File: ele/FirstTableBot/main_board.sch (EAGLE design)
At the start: 164 parts, among them IC3 CP2102N-28, T1 BC337, T2 BC337, U1 ESP-WROOM-32, U2 UM18533, X3 USB-MICRO-B-BOTTOM, X4 POWER_IN

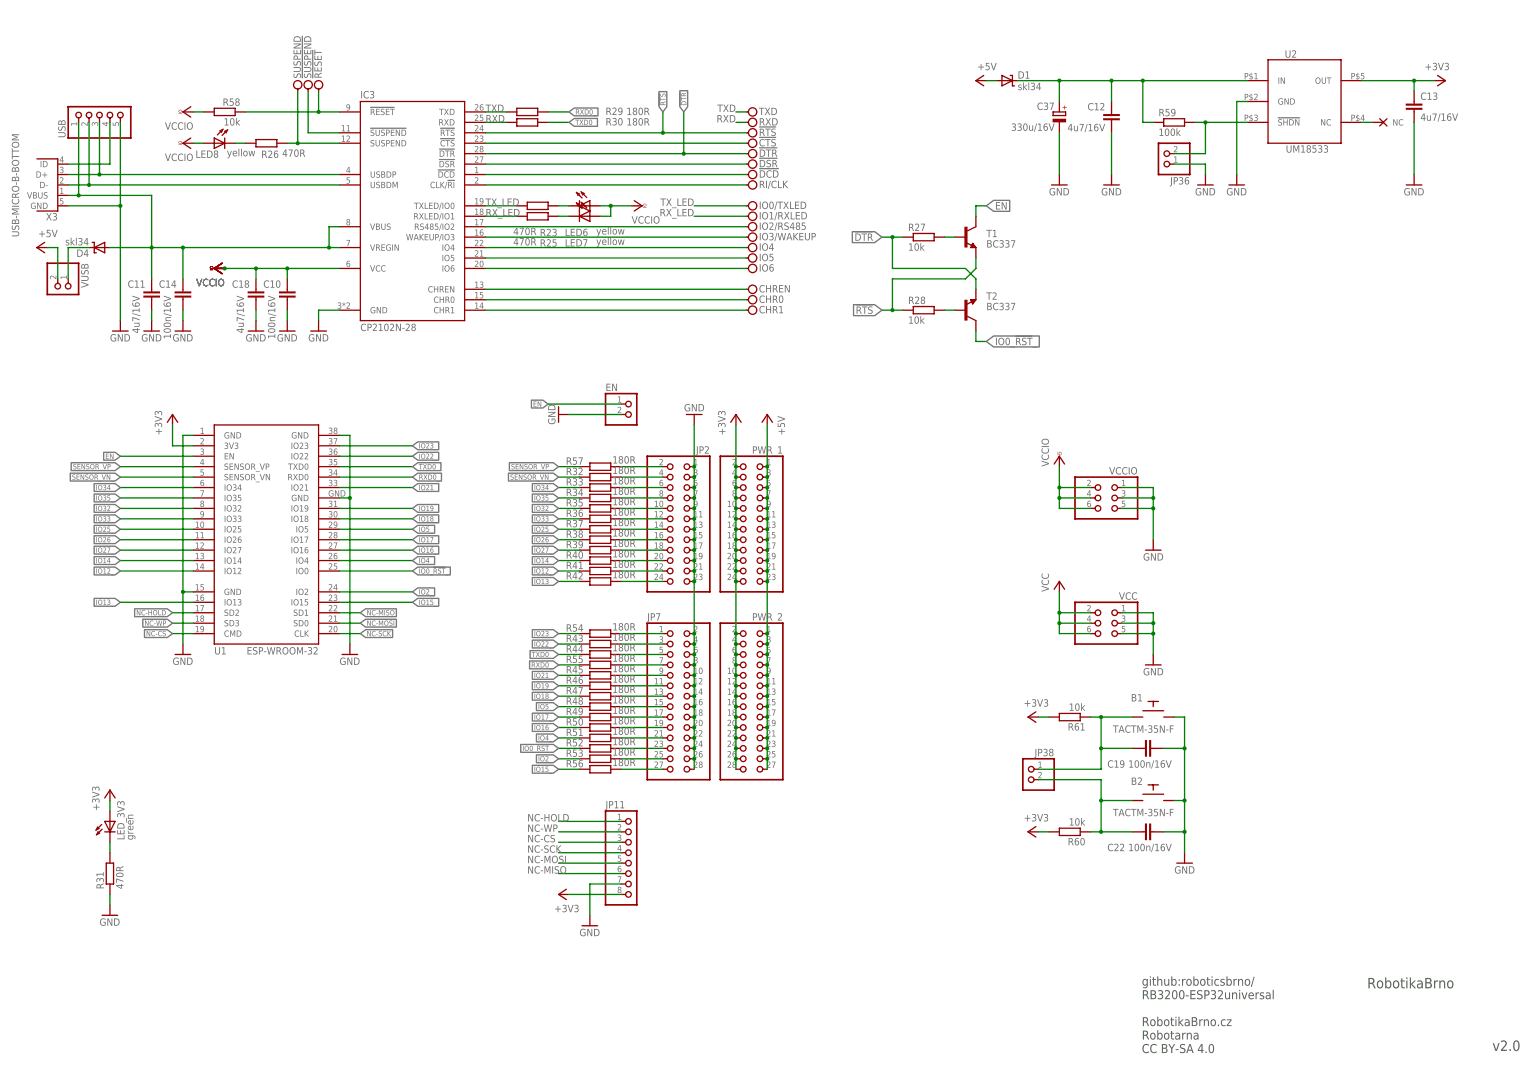
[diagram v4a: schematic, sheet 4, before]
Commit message: mereni proudu
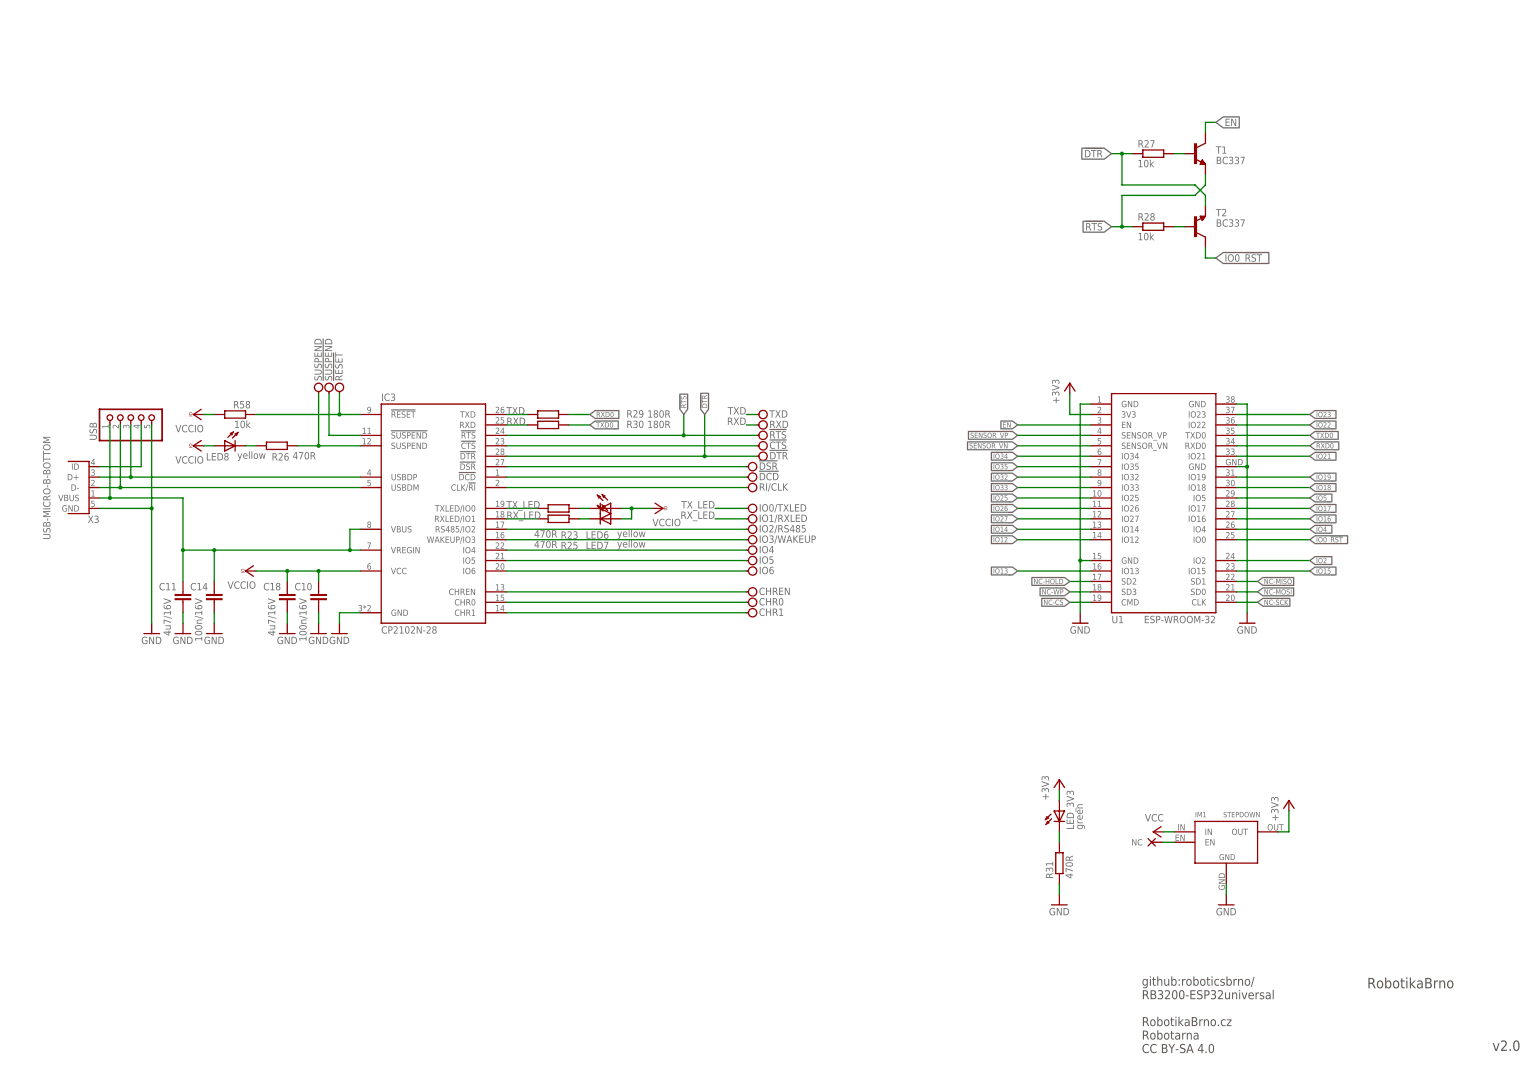
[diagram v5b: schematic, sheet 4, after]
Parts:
- removed B1, B2: TACTM-35N-F, TACTM-35N-F:TACTM-35N-F
- removed C12, C13: 4u7/16V, rcl_upravena:C-EUC0603
- removed C19, C22: 100n/16V, rcl_upravena:C-EUC0402
- removed C37: 330u/16V, rcl_upravena:CPOL-EUE5-10.5
- removed D1, D4: skl34, diode:SHOTTKY-SOD123
- removed EN, JP36, JP38, VUSB: (no value), pinhead:PINHD-1X2
- removed JP11: (no value), pinhead:PINHD-1X8
- removed JP2, PWR_1: (no value), pinhead:PINHD-2X12
- removed JP7, PWR_2: (no value), pinhead:PINHD-2X14
- removed NC7: NC, NC:NC
- removed R32, R33, R34, R35, R36, R37, R38, R39, R40, R41, R42, R43, R44, R45, R46, R47, R48, R49, R50, R51, R52, R53, R54, R55, R56, R57: 180R, rcl_upravena:R-EU_R0603
- removed R59: 100k, rcl_upravena:R-EU_R0603
- removed R60, R61: 10k, rcl_upravena:R-EU_R0603
- removed U2: UM18533, um185xx:UM185XX
- removed VCC, VCCIO: (no value), pinhead:PINHD-2X3
- added IM1: STEPDOWN, StepDown:STEPDOWN
- added NC2: NC, NC:NC
- added R19, R62: (no value), resistor:R-EU_M1206
- added U$11: BA10358F-E2SOIC, Rohm:BA10358F-E2SOIC
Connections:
- removed net !SHDN: JP36.2, R59.2, U2.!SHDN
- removed net 3V3_IN: C12.1, C37.+, D1.C, R59.1, U2.IN
- removed net 5V_USB: D4.C, VUSB.1
- removed net BTN0: B1.P$4, C19.2, JP38.1, R61.1
- removed net BTN1: B2.P$4, C22.2, JP38.2, R60.1
- removed net IO0_!RST: JP7.23, R52.1
- removed net IO12: JP2.22, R41.1
- removed net IO13: JP2.24, R42.1
- removed net IO14: JP2.20, R40.1
- removed net IO15: JP7.27, R56.1
- removed net IO16: JP7.19, R50.1
- removed net IO17: JP7.17, R49.1
- removed net IO18: JP7.13, R47.1
- removed net IO19: JP7.11, R46.1
- removed net IO2: JP7.25, R53.1
- removed net IO21: JP7.9, R45.1
- removed net IO22: JP7.3, R43.1
- removed net IO23: JP7.1, R54.1
- removed net IO25: JP2.14, R37.1
- removed net IO26: JP2.16, R38.1
- removed net IO27: JP2.18, R39.1
- removed net IO32: JP2.10, R35.1
- removed net IO33: JP2.12, R36.1
- removed net IO34: JP2.6, R33.1
- removed net IO35: JP2.8, R34.1
- removed net IO4: JP7.21, R51.1
- removed net IO5: JP7.15, R48.1
- removed net RXD0: JP7.7, R55.1
- removed net SENSOR_VN: JP2.4, R32.1
- removed net SENSOR_VP: JP2.2, R57.1
- removed net TXD0: JP7.5, R44.1
- removed net U2_NC: NC7.NC, U2.NC
- new net AMPLIFIED_I-MOT_A: U$11.OUT2
- new net AMPLIFIED_I-MOT_B: U$11.OUT1
- new net I-MOT_A: R19.2, U$11.+IN2, U$9.AISEN
- new net I-MOT_B: R62.2, U$11.+IN1, U$9.BISEN
- new net IO9_NC1: IM1.EN, NC2.NC
- net +3V3: now also IM1.OUT; no longer C13.1, JP11.8, PWR_1.10, PWR_1.12, PWR_1.14, PWR_1.16, PWR_1.18, PWR_1.2, PWR_1.20, PWR_1.22, PWR_1.24, PWR_1.4, PWR_1.6, PWR_1.8, PWR_2.10, PWR_2.12, PWR_2.14, PWR_2.16, PWR_2.18, PWR_2.2, PWR_2.20, PWR_2.22, PWR_2.24, PWR_2.26, PWR_2.28, PWR_2.4, PWR_2.6, PWR_2.8, R60.2, R61.2, U2.OUT
- net +5V: no longer D1.A, PWR_1.1, PWR_1.11, PWR_1.13, PWR_1.15, PWR_1.17, PWR_1.19, PWR_1.21, PWR_1.23, PWR_1.3, PWR_1.5, PWR_1.7, PWR_1.9, PWR_2.1, PWR_2.11, PWR_2.13, PWR_2.15, PWR_2.17, PWR_2.19, PWR_2.21, PWR_2.23, PWR_2.25, PWR_2.27, PWR_2.3, PWR_2.5, PWR_2.7, PWR_2.9, VUSB.2
- net EN: no longer EN.1
- net GND: now also IM1.GND, R19.1, R62.1, U$11.-IN1, U$11.-IN2, U$11.VEE; no longer B1.P$3, B2.P$3, C12.2, C13.2, C19.1, C22.1, C37.-, EN.2, JP11.7, JP2.1, JP2.11, JP2.13, JP2.15, JP2.17, JP2.19, JP2.21, JP2.23, JP2.3, JP2.5, JP2.7, JP2.9, JP36.1, JP7.10, JP7.12, JP7.14, JP7.16, JP7.18, JP7.2, JP7.20, JP7.22, JP7.24, JP7.26, JP7.28, JP7.4, JP7.6, JP7.8, U$9.AISEN, U$9.BISEN, U2.GND, VCC.1, VCC.3, VCC.5, VCCIO.1, VCCIO.3, VCCIO.5
- net IO0_!RST!_: no longer R52.2
- net IO12_: no longer R41.2
- net IO13_: no longer R42.2
- net IO14_: no longer R40.2
- net IO15_: no longer R56.2
- net IO16_: no longer R50.2
- net IO17_: no longer R49.2
- net IO18_: no longer R47.2
- net IO19_: no longer R46.2
- net IO21_: no longer R45.2
- net IO22_: no longer R43.2
- net IO23_: no longer R54.2
- net IO25_: no longer R37.2
- net IO26_: no longer R38.2
- net IO27_: no longer R39.2
- net IO2_: no longer R53.2
- net IO32_: no longer R35.2
- net IO33_: no longer R36.2
- net IO34_: no longer R33.2
- net IO35_: no longer R34.2
- net IO4_: no longer R51.2
- net IO5_: no longer R48.2
- net NC-CS: no longer JP11.3
- net NC-HOLD: no longer JP11.1
- net NC-MISO: no longer JP11.6
- net NC-MOSI: no longer JP11.5
- net NC-SCK: no longer JP11.4
- net NC-WP: no longer JP11.2
- net RXD0_: no longer R55.2
- net SENSOR_VN_: no longer R32.2
- net SENSOR_VP_: no longer R57.2
- net TXD0_: no longer R44.2
- net VCC: now also IM1.IN, U$11.VCC; no longer VCC.2, VCC.4, VCC.6
- net VCCIO: no longer VCCIO.2, VCCIO.4, VCCIO.6
- net VUSB: no longer D4.A
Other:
- moved on the sheet: C10, C11, C14, C18, C23, C6, C7, CHR0, CHR1, CHREN, D3, IC3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

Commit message: ir led pro encodery
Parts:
- removed !CTS, !DCD, !DSR, !DTR, !RESET, !RTS, !SUSPEND, CHR0, CHR1, CHREN, IO0/TXLED, IO1/RXLED, IO2/RS485, IO3/WAKEUP, IO4, IO5, IO6, RI/CLK, RXD, SUSPEND, TXD: PINH1X01, pinhead_smd:PINH1X01
- removed C10, C14: 100n/16V, rcl_upravena:C-EUC0402
- removed C11, C18: 4u7/16V, rcl_upravena:C-EUC0603
- removed IC3: CP2102N-28, CP2102N:CP2102N-28
- removed IM1: STEPDOWN, StepDown:STEPDOWN
- removed JP1: PINH2X06, pinhead_smd:PINH2X06
- removed LED6, LED7, LED8: yellow, led:LEDCHIP-LED0603
- removed LED_3V3: green, led:LEDCHIPLED_0603
- removed NC2: NC, NC:NC
- removed R29, R30: 180R, rcl_upravena:R-EU_R0603
- removed R31: 470R, rcl_upravena:R-EU_R0603
- removed R58: 10k, rcl_upravena:R-EU_R0603
- removed RN1: (no value), resistor-dil:2R-NEXB24V
- removed T1, T2: BC337, transistors:NPN-SOT23-BEC
- removed U1: ESP-WROOM-32, esp32:ESP-WROOM-32
- removed USB: (no value), pinhead:PINHD-1X5
- removed X3: USB-MICRO-B-BOTTOM, usb:USB-MICRO-B-BOTTOM
- added D2: (no value), diode:DIODE-D-7.5
- added IM6: DEVKITC, esp32:DEVKITC
- added JP2: (no value), pinhead:PINHD-1X6
- added R32, R33, R34, R35: (no value), resistor:R-EU_R0603
- added U$10, U$12, U$13, U$14: L-NP-3C1, led-brt:L-NP-3C1
- added U$16, U$17, U$18, U$19: BIR-NM13C1, led-brt:BIR-NM13C1
- LED0, LED1, LED2, LED3, LED4: device led:LED3MM -> led:LEDCHIPLED_1206
- LED5: value BLUE -> GREEN
- Q2, Q5: device transistors:P-MOSFET-TO220V -> transistors:P-MOSFET-MLP_HS
- R19, R62: device resistor:R-EU_M1206 -> resistor:R-EU_R0603
- R23: value 470R -> (none); device rcl_upravena:R-EU_R0603 -> resistor:R-EU_R0805
- R25, R26: value 470R -> (none); device rcl_upravena:R-EU_R0603 -> resistor:R-EU_R0603
- R27, R28: value 10k -> (none); device rcl_upravena:R-EU_R0603 -> resistor:R-EU_R0603
- RN2: device resistor-dil:4R-N0402ARV341 -> resistor-dil:4R-NEXBS8V
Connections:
- removed net !DTR: !DTR.1, IC3.!DTR, R27.1, T2.E
- removed net !DTR_B: R27.2, T1.B
- removed net !RESET: !RESET.1, IC3.!RESET, R58.1
- removed net !RTS: !RTS.1, IC3.!RTS, R28.1, T1.E
- removed net !RTS_B: R28.2, T2.B
- removed net !SUSPEND: !SUSPEND.1, IC3.!SUSPEND
- removed net CHR0: CHR0.1, IC3.CHR0
- removed net CHR1: CHR1.1, IC3.CHR1
- removed net CHREN: CHREN.1, IC3.CHREN
- removed net CLK/!RI: IC3.CLK/!RI, RI/CLK.1
- removed net DCD: !DCD.1, IC3.!DCD
- removed net DM: IC3.USBDM, USB.2, X3.D-
- removed net DP: IC3.USBDP, USB.3, X3.D+
- removed net DSR: !DSR.1, IC3.!DSR
- removed net EN: T1.C, U1.EN
- removed net IO0_!RST!_: T2.C, U1.IO0
- removed net IO12_: U1.IO12
- removed net IO13_: U1.IO13
- removed net IO14_: U1.IO14
- removed net IO15_: U1.IO15
- removed net IO16_: U1.IO16
- removed net IO17_: U1.IO17
- removed net IO18_: U1.IO18
- removed net IO19_: U1.IO19
- removed net IO21_: U1.IO21
- removed net IO22_: U1.IO22
- removed net IO23_: U1.IO23
- removed net IO25_: U1.IO25
- removed net IO26_: U1.IO26
- removed net IO27_: U1.IO27
- removed net IO2_: U1.IO2
- removed net IO32_: U1.IO32
- removed net IO33_: U1.IO33
- removed net IO34_: U1.IO34
- removed net IO35_: U1.IO35
- removed net IO4_: U1.IO4
- removed net IO5_: U1.IO5
- removed net IO9_NC1: IM1.EN, NC2.NC
- removed net LED_3V3: LED_3V3.C, R31.2
- removed net N$24: U$8.PB2/GPIO/CLK
- removed net NC-CS: U1.CMD
- removed net NC-HOLD: U1.SD2
- removed net NC-MISO: U1.SD1
- removed net NC-MOSI: U1.SD0
- removed net NC-SCK: U1.CLK
- removed net NC-WP: U1.SD3
- removed net PWM_A2: U$9.AIN2
- removed net PWM_B2: U$9.BIN2
- removed net RX-LED: LED7.C, R25.1
- removed net RXD: IC3.RXD, R30.1, RXD.1
- removed net RXD0_: R29.2, U1.RXD0
- removed net RX_LED: IC3.RXLED/IO1, IO1/RXLED.1, R25.2
- removed net SENSOR_VN_: U1.SENSOR_VN
- removed net SENSOR_VP_: U1.SENSOR_VP
- removed net SUSPEND: IC3.SUSPEND, R26.1, SUSPEND.1
- removed net TX-LED: LED6.C, R23.1
- removed net TXD: IC3.TXD, R29.1, TXD.1
- removed net TXD0_: R30.2, U1.TXD0
- removed net TX_LED: IC3.TXLED/IO0, IO0/TXLED.1, R23.2
- removed net USBID: USB.4, X3.ID
- removed net USBIO3_RS485: IC3.RS485/IO2, IO2/RS485.1
- removed net USBIO3_WAKEUP: IC3.WAKEUP/IO3, IO3/WAKEUP.1
- removed net USBIO4: IC3.IO4, IO4.1
- removed net USBIO5: IC3.IO5, IO5.1
- removed net USBIO6: IC3.IO6, IO6.1
- removed net VCCIO: C10.1, C18.1, IC3.VCC, LED6.A, LED7.A, LED8.A, R58.2
- removed net VUSB: C11.1, C14.1, IC3.VBUS, IC3.VREGIN, USB.1, X3.VBUS
- new net +5V_ESP: D2.C, IM6.5V
- new net CDA: IM6.IO2, U$8.PB2/GPIO/CLK
- new net ENC-A0: IM6.SVP, R32.2, U$10.PIN
- new net ENC-A1: IM6.SVN, R33.2, U$12.PIN
- new net ENC-B0: IM6.IO34, R34.2, U$13.PIN
- new net ENC-B1: IM6.IO35, R35.2, U$14.PIN
- new net N$18: R26.2, U$17.VCC
- new net N$19: R27.2, U$18.VCC
- new net N$20: R28.2, U$19.VCC
- new net PWM_A0: IM6.IO12, U$9.AIN1
- new net PWM_B0: IM6.IO17, U$9.BIN1
- net +3V3: now also IM6.3V3; no longer IM1.OUT, LED_3V3.A, U1.3V3
- net +5V: now also D2.A, JP2.2, R25.1, R26.1, R27.1, R28.1, R32.1, R33.1, R34.1, R35.1; no longer JP1B2.1, JP1T2.1
- net GND: now also IM6.GND, JP2.3, U$10.GND, U$12.GND, U$13.GND, U$14.GND, U$16.GND, U$17.GND, U$18.GND, U$19.GND; no longer C1.2, C10.2, C11.2, C14.2, C18.2, IC3.GND, IM1.GND, JP1B3.1, JP1T3.1, R18.2, R31.1, SW4.P, SW4.P1, U1.GND@1, U1.GND@2, U1.GND@3, U1.GND@4, USB.5, X3.GND
- net MISO: now also JP2.5; no longer JP1B5.1, JP1T5.1
- net MOSI: now also JP2.6; no longer JP1B6.1, JP1T6.1
- net N$12: now also R25.2, U$16.VCC; no longer !CTS.1, IC3.!CTS
- net N$13: now also C1.2, R18.2, SW4.P, SW4.P1; no longer LED8.C, R26.2
- net PB3: now also R23.1; no longer RN1A.1
- net PWM_A1: now also IM6.IO16, U$9.AIN2; no longer U$9.AIN1
- net PWM_B1: now also IM6.IO5, U$9.BIN2; no longer U$9.BIN1
- net RESET: now also JP2.1; no longer JP1B1.1, JP1T1.1
- net SCK: now also IM6.IO0, JP2.4; no longer JP1B4.1, JP1T4.1
- net SW4: now also R23.2; no longer RN1A.2
- net VCC: no longer IM1.IN
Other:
- note removed: "RobotikaBrno"
- note removed: "github:roboticsbrno/ RB3200-ESP32universal RobotikaBrno.cz Robotarna CC BY-SA 4.0"
- note removed: "v2.0"
